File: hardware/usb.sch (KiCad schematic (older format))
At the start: 2 parts

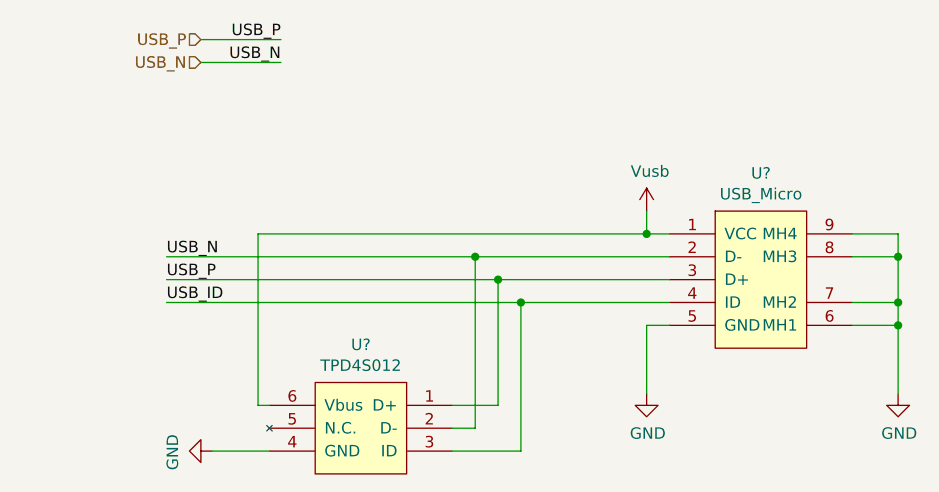
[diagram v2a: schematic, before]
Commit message: update,
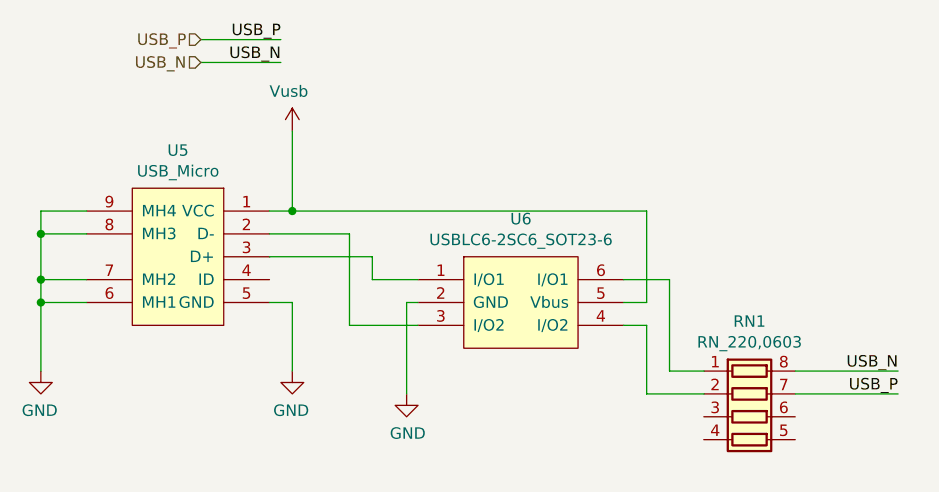
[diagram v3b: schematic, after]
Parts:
- removed U?: TPD4S012, footprints-lib:TPD4S012, symbol taobao-components:TPD4S012
- added RN1: RN_220,0603, Resistor_SMD:R_Array_Concave_4x0603, symbol taobao-rpack:RN_220,0603
- added U6: USBLC6-2SC6_SOT23-6, footprints-lib:USBLC6-2, symbol taobao-components:USBLC6-2SC6_SOT23-6
- gave numbers to parts that had none: 1
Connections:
- net GND: now also U6.2 (GND)
- net USB_N: now also RN1.8 (R1.2); no longer U5.2 (D-)
- net USB_P: now also RN1.7 (R2.2); no longer U5.3 (D+)
- net Vusb: now also U6.5 (Vbus)
- net USB_ID: no longer names the net of U5.4 (ID)
- new net: U5.2 (D-), U6.3 (I/O2)
- new net: U5.3 (D+), U6.1 (I/O1)
- new net: RN1.2 (R2.1), U6.4 (I/O2)
- new net: RN1.1 (R1.1), U6.6 (I/O1)
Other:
- moved on the sheet: U5
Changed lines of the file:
@@
 $EndDescr
 $Comp
-L taobao-components:USB_Micro U?
+L taobao-components:USB_Micro U5
 U 1 1 5D0A4A6D
-P 3850 1800
-F 0 "U?" H 3850 2265 50  0000 C CNN
-F 1 "USB_Micro" H 3850 2174 50  0000 C CNN
-F 2 "footprint-lib:USB_Micro-B_Molex-105017-0001" H 3850 1300 50  0001 C CNN
-F 3 "" H 3850 1300 50  0001 C CNN
-	1    3850 1800
-	1    0    0    -1
+P 1300 1700
+F 0 "U5" H 1300 2165 50  0000 C CNN
+F 1 "USB_Micro" H 1300 2074 50  0000 C CNN
+F 2 "footprint-lib:USB_Micro-B_Molex-105017-0001" H 1300 1200 50  0001 C CNN
+F 3 "" H 1300 1200 50  0001 C CNN
+	1    1300 1700
+	-1   0    0    -1
 $EndComp
 $Comp
-L power:GND #PWR?
+L power:GND #PWR0116
 U 1 1 5D0A4EF1
-P 4450 2300
-F 0 "#PWR?" H 4450 2050 50  0001 C CNN
-F 1 "GND" H 4455 2127 50  0000 C CNN
-F 2 "" H 4450 2300 50  0001 C CNN
-F 3 "" H 4450 2300 50  0001 C CNN
-	1    4450 2300
-	1    0    0    -1
+P 700 2200
+F 0 "#PWR0116" H 700 1950 50  0001 C CNN
+F 1 "GND" H 705 2027 50  0000 C CNN
+F 2 "" H 700 2200 50  0001 C CNN
+F 3 "" H 700 2200 50  0001 C CNN
+	1    700  2200
+	-1   0    0    -1
 $EndComp
 Wire Wire Line
-	4250 1600 4450 1600
+	900  1500 700  1500
 Wire Wire Line
-	4450 1600 4450 1700
+	700  1500 700  1600
 Wire Wire Line
-	4250 1700 4450 1700
-Connection ~ 4450 1700
+	900  1600 700  1600
+Connection ~ 700  1600
 Wire Wire Line
-	4450 1700 4450 1900
+	700  1600 700  1800
 Wire Wire Line
-	4250 1900 4450 1900
-Connection ~ 4450 1900
+	900  1800 700  1800
+Connection ~ 700  1800
 Wire Wire Line
-	4450 1900 4450 2000
+	700  1800 700  1900
 Wire Wire Line
-	4250 2000 4450 2000
-Connection ~ 4450 2000
+	900  1900 700  1900
+Connection ~ 700  1900
 Wire Wire Line
-	4450 2000 4450 2300
+	700  1900 700  2200
 $Comp
-L power:GND #PWR?
+L power:GND #PWR0117
 U 1 1 5D0A5204
-P 3350 2300
-F 0 "#PWR?" H 3350 2050 50  0001 C CNN
-F 1 "GND" H 3355 2127 50  0000 C CNN
-F 2 "" H 3350 2300 50  0001 C CNN
-F 3 "" H 3350 2300 50  0001 C CNN
-	1    3350 2300
-	1    0    0    -1
+P 1800 2200
+F 0 "#PWR0117" H 1800 1950 50  0001 C CNN
+F 1 "GND" H 1805 2027 50  0000 C CNN
+F 2 "" H 1800 2200 50  0001 C CNN
+F 3 "" H 1800 2200 50  0001 C CNN
+	1    1800 2200
+	-1   0    0    -1
 $EndComp
 Wire Wire Line
-	3350 2300 3350 2000
+	1800 2200 1800 1900
 Wire Wire Line
-	3350 2000 3450 2000
+	1800 1900 1700 1900
 Text HLabel 1400 750  0    50   Input ~ 0
 USB_P
@@
 Wire Wire Line
 	1400 850  1750 850
-Text Label 1250 1800 0    50   ~ 0
-USB_P
-Text Label 1250 1700 0    50   ~ 0
-USB_N
 Wire Wire Line
-	3450 1600 3350 1600
+	1700 1500 1800 1500
 Wire Wire Line
-	3350 1600 3350 1500
+	1800 1500 1800 1150
 $Comp
-L my_power:Vusb #PWR?
+L my_power:Vusb #PWR0115
 U 1 1 5D0A9977
-P 3350 1500
-F 0 "#PWR?" H 3350 1350 50  0001 C CNN
-F 1 "Vusb" H 3365 1673 50  0000 C CNN
-F 2 "" H 3350 1500 50  0001 C CNN
-F 3 "" H 3350 1500 50  0001 C CNN
-	1    3350 1500
-	1    0    0    -1
-$EndComp
-$Comp
-L taobao-components:TPD4S012 U?
-U 1 1 5D0B5624
-P 2100 2450
-F 0 "U?" H 2100 2815 50  0000 C CNN
-F 1 "TPD4S012" H 2100 2724 50  0000 C CNN
-F 2 "footprints-lib:TPD4S012" H 2100 2400 50  0001 C CNN
-F 3 "" H 2100 2400 50  0001 C CNN
-	1    2100 2450
+P 1800 1150
+F 0 "#PWR0115" H 1800 1000 50  0001 C CNN
+F 1 "Vusb" H 1815 1323 50  0000 C CNN
+F 2 "" H 1800 1150 50  0001 C CNN
+F 3 "" H 1800 1150 50  0001 C CNN
+	1    1800 1150
 	-1   0    0    -1
 $EndComp
-Text Label 1250 1900 0    50   ~ 0
-USB_ID
-$Comp
-L power:GND #PWR?
-U 1 1 5D0BBCB3
-P 1450 2550
-F 0 "#PWR?" H 1450 2300 50  0001 C CNN
-F 1 "GND" H 1455 2377 50  0000 C CNN
-F 2 "" H 1450 2550 50  0001 C CNN
-F 3 "" H 1450 2550 50  0001 C CNN
-	1    1450 2550
-	0    1    1    0
-$EndComp
-Wire Wire Line
-	1450 2550 1700 2550
-Wire Wire Line
-	3350 1600 1650 1600
-Wire Wire Line
-	1650 1600 1650 2350
-Wire Wire Line
-	1650 2350 1700 2350
-Connection ~ 3350 1600
-Wire Wire Line
-	1250 1800 2700 1800
-Wire Wire Line
-	1250 1700 2600 1700
-Wire Wire Line
-	1250 1900 2800 1900
-Wire Wire Line
-	2500 2450 2600 2450
-Wire Wire Line
-	2600 2450 2600 1700
-Connection ~ 2600 1700
-Wire Wire Line
-	2600 1700 3450 1700
-Wire Wire Line
-	2700 1800 2700 2350
-Wire Wire Line
-	2700 2350 2500 2350
-Connection ~ 2700 1800
-Wire Wire Line
-	2700 1800 3450 1800
-Wire Wire Line
-	2800 1900 2800 2550
-Wire Wire Line
-	2800 2550 2500 2550
-Connection ~ 2800 1900
-Wire Wire Line
-	2800 1900 3450 1900
 $Bitmap
 Pos -850 1900
@@
 EndData
 $EndBitmap
+Wire Wire Line
+	1700 1600 2050 1600
+Wire Wire Line
+	1700 1700 2150 1700
+$Comp
+L taobao-components:USBLC6-2SC6_SOT23-6 U6
+U 1 1 5D3156EE
+P 2800 1900
+F 0 "U6" H 2800 2265 50  0000 C CNN
+F 1 "USBLC6-2SC6_SOT23-6" H 2800 2174 50  0000 C CNN
+F 2 "footprints-lib:USBLC6-2" H 2800 1400 50  0001 C CNN
+F 3 "" H 2800 1850 50  0001 C CNN
+	1    2800 1900
+	1    0    0    -1
+$EndComp
+Wire Wire Line
+	2350 2000 2050 2000
+Wire Wire Line
+	2050 2000 2050 1600
+Wire Wire Line
+	2350 1800 2150 1800
+Wire Wire Line
+	2150 1800 2150 1700
+Wire Wire Line
+	1800 1500 3350 1500
+Wire Wire Line
+	3350 1500 3350 1900
+Wire Wire Line
+	3350 1900 3250 1900
+Connection ~ 1800 1500
+$Comp
+L taobao-rpack:RN_220,0603 RN1
+U 1 1 5D31870E
+P 3800 2400
+F 0 "RN1" V 3383 2400 50  0000 C CNN
+F 1 "RN_220,0603" V 3474 2400 50  0000 C CNN
+F 2 "Resistor_SMD:R_Array_Concave_4x0603" V 4075 2400 50  0001 C CNN
+F 3 "~" H 3800 2400 50  0001 C CNN
+	1    3800 2400
+	0    1    1    0
+$EndComp
+Wire Wire Line
+	3250 1800 3450 1800
+Wire Wire Line
+	3450 1800 3450 2200
+Text Label 4450 2300 2    50   ~ 0
+USB_P
+Text Label 4450 2200 2    50   ~ 0
+USB_N
+Wire Wire Line
+	4000 2200 4450 2200
+Wire Wire Line
+	4000 2300 4450 2300
+Wire Wire Line
+	3450 2200 3600 2200
+Wire Wire Line
+	3250 2000 3350 2000
+Wire Wire Line
+	3350 2000 3350 2300
+Wire Wire Line
+	3350 2300 3600 2300
+$Comp
+L power:GND #PWR0118
+U 1 1 5D3240FA
+P 2300 2300
+F 0 "#PWR0118" H 2300 2050 50  0001 C CNN
+F 1 "GND" H 2305 2127 50  0000 C CNN
+F 2 "" H 2300 2300 50  0001 C CNN
+F 3 "" H 2300 2300 50  0001 C CNN
+	1    2300 2300
+	1    0    0    -1
+$EndComp
+Wire Wire Line
+	2300 2300 2300 1900
+Wire Wire Line
+	2300 1900 2350 1900
 $EndSCHEMATC
